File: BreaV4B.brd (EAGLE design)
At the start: 30.8 x 19 mm, 32 parts, among them J1 XF2L-0535-1, J2 XF2L-0535-1, Q3 ABM-16MHZ, SW1 ESE31L11T, SW2 EVQ11U09K, SW3 LS12T2-T, U1 TPS62200, X1 22-23-2021

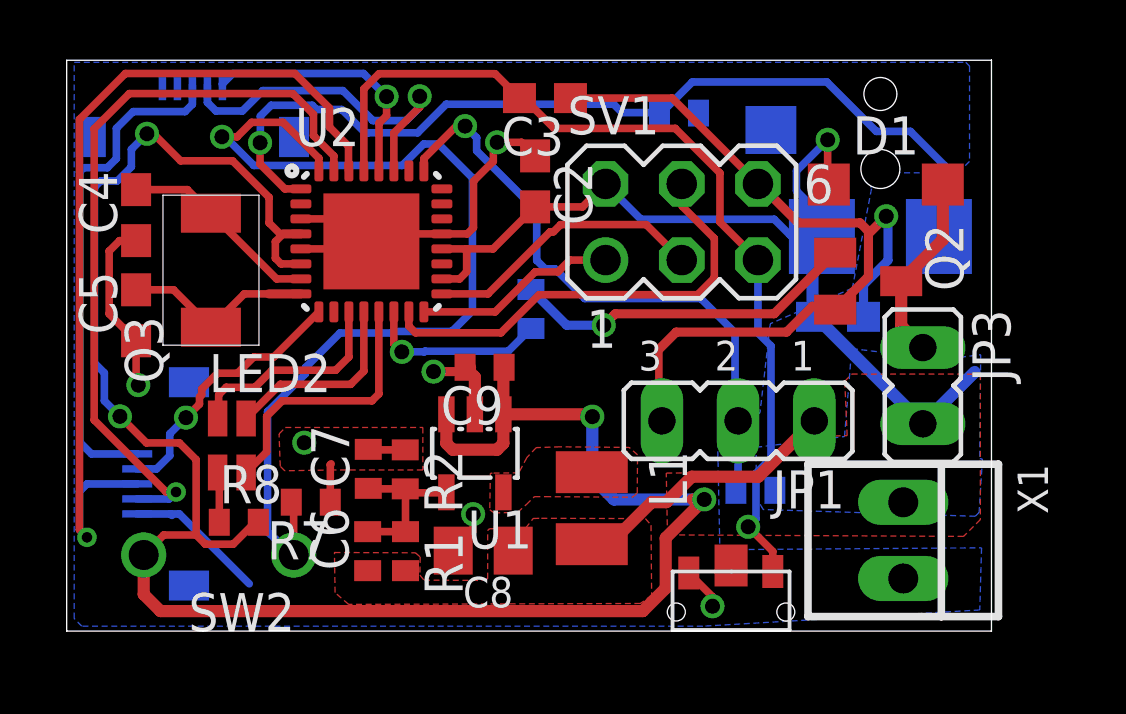
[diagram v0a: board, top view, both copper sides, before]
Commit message: Rx Tx
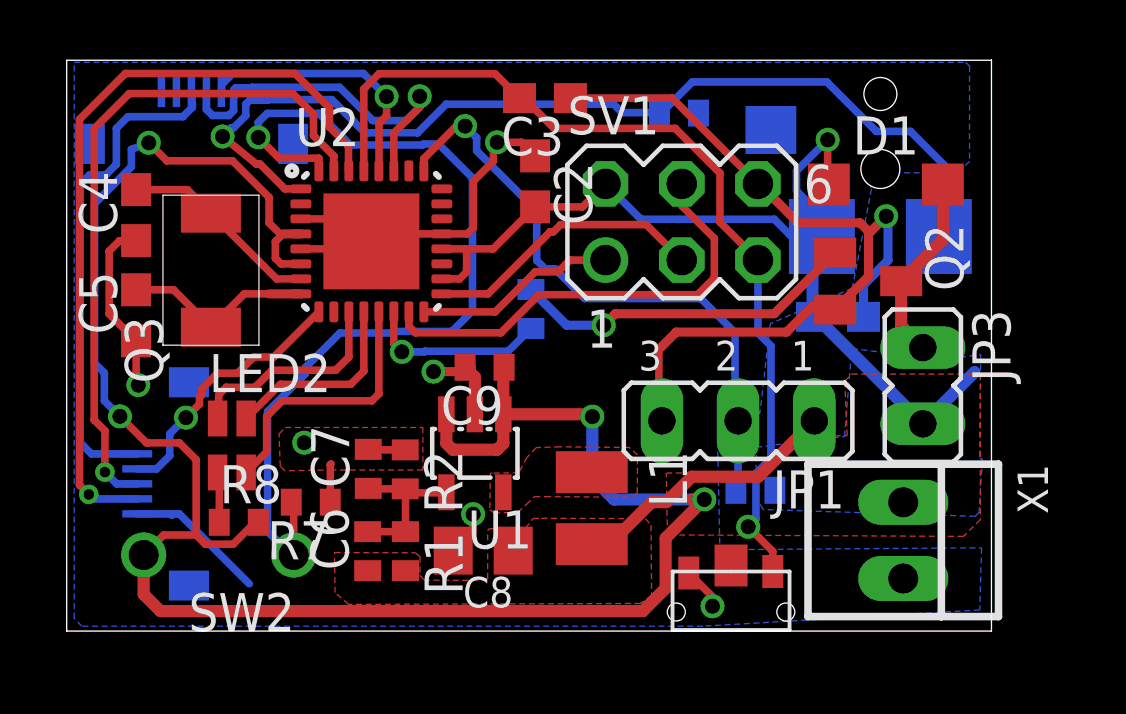
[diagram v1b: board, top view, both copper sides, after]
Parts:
- moved J2 0.23 mm to (4.16, 16.0)
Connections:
- net RX: now also J1.4; no longer J1.3
- net TX: now also J1.3; no longer J1.4
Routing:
- net RX: track 29.5 -> 26.1 mm
- net PWRSW: track 33.6 -> 31.1 mm
- net TX: track 25.1 -> 23.1 mm
- net DETSW: track 31.2 -> 33.1 mm
- net VCC: track 100.4 -> 99.8 mm
- net SDA: track 11.9 -> 12.4 mm
